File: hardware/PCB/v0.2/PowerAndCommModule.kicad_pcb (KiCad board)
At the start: 2 copper layers, 39.7 x 52.1 mm, 18 parts, among them J1 Screw_Terminal_01x02, J2 Conn_01x06_Pin, J3 Screw_Terminal_01x02, J4 Conn_01x04_Socket, J5 Screw_Terminal_01x02, K1 HF49FD_005-1H22G, Q1 S8050, SW1 SW_DIP_x01, U1 AMS1117-3.3, U2 ESP-32s

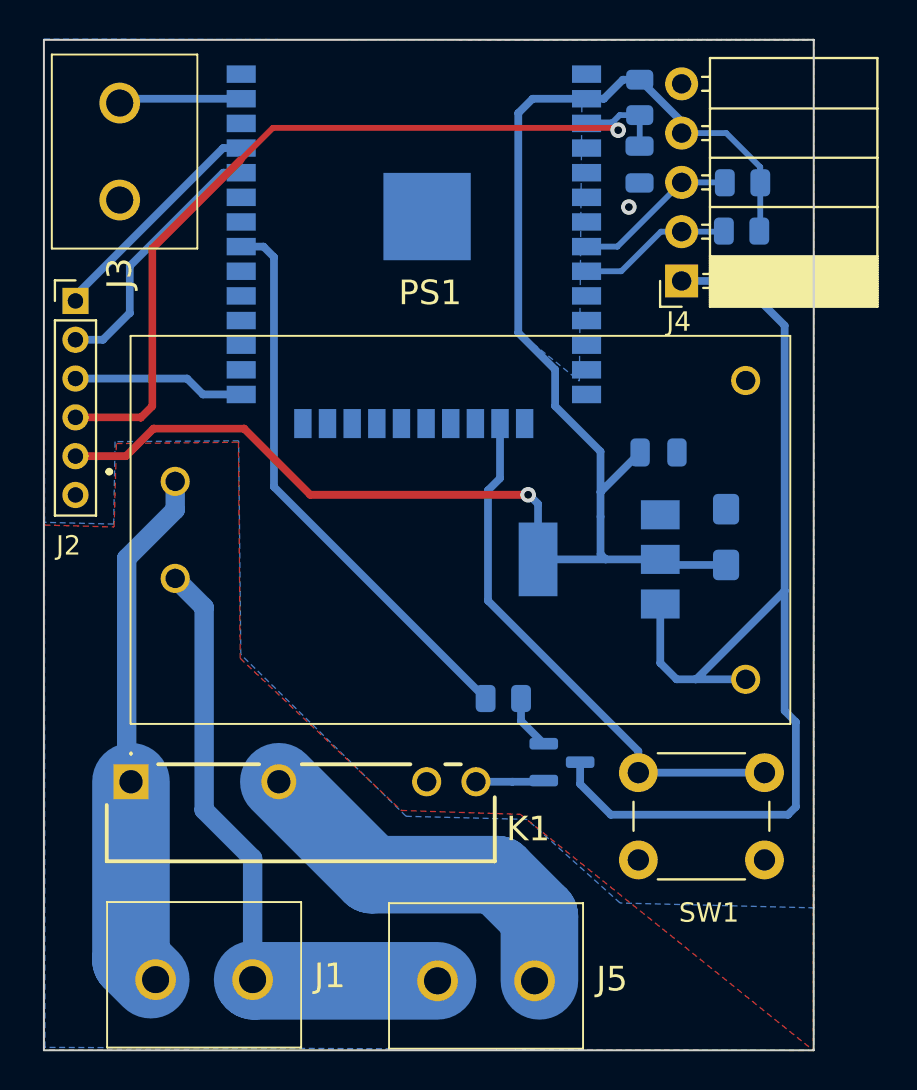
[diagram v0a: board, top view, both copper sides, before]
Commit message: commit before system update
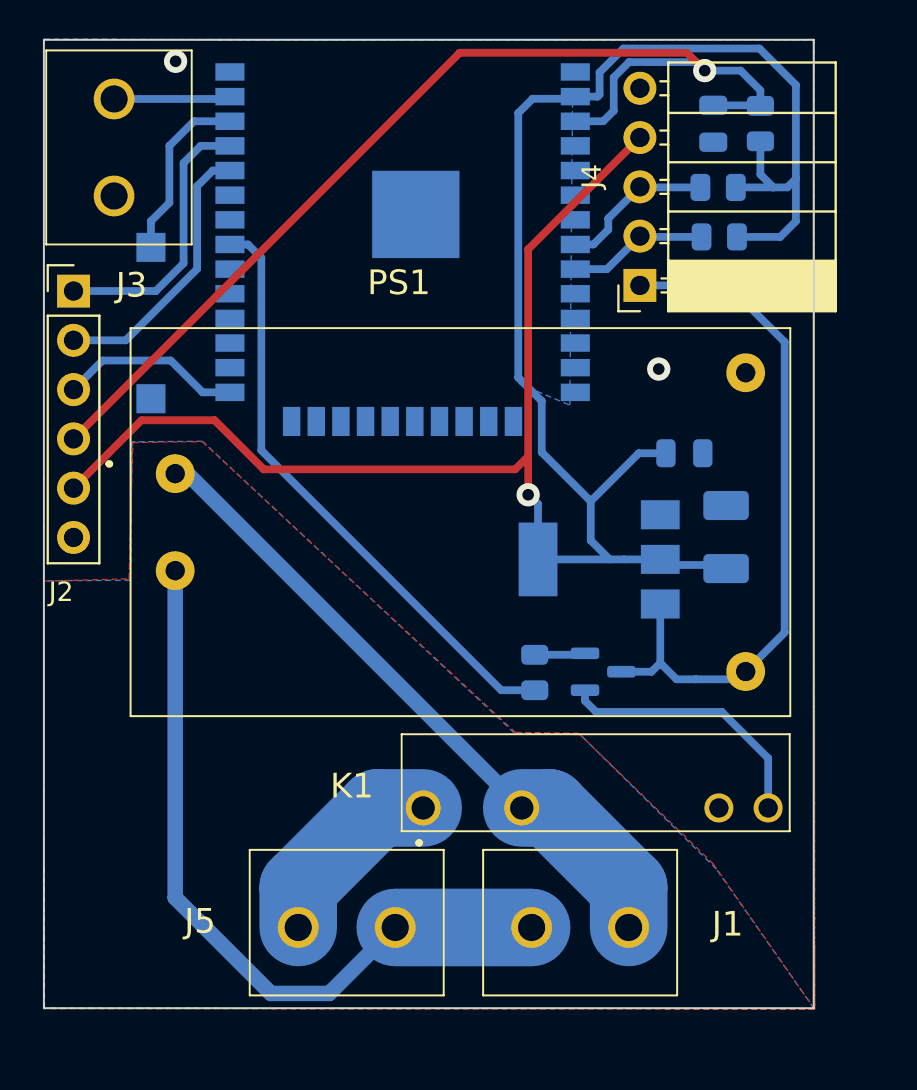
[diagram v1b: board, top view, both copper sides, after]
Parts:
- C1: footprint Capacitor_Tantalum_SMD:CP_EIA-3216-18_Kemet-A_Pad1.58x1.35mm_HandSolder -> Capacitor_Tantalum_SMD:CP_EIA-3528-21_Kemet-B_Pad1.50x2.35mm_HandSolder
- J2: footprint Connector_PinHeader_2.00mm:PinHeader_1x06_P2.00mm_Vertical -> Connector_PinHeader_2.54mm:PinHeader_1x06_P2.54mm_Vertical
- K1: value HF49FD_005-1H22G -> HF49FD_005-1H11G; footprint HF49FD_005:HF49FD0051H22G -> HF49FD_005-1H11:HF49FD0051H11F
- SW1: footprint Button_Switch_THT:SW_PUSH_6mm_H4.3mm -> Button_Switch_SMD:SW_SPST_CK_RS282G05A3; moved to B.Cu
- moved SW1 34.2 mm to (31.8, 42.6), turned to -90 degrees
- moved K1 24.0 mm to (54.7, 66.7)
- moved J1 19.6 mm to (51.4, 73.8)
- moved J5 7.69 mm to (39.4, 73.8)
- moved R1 6.36 mm to (63.2, 32.3), turned to 90 degrees
- moved Q1 5.12 mm to (55.1, 60.6)
- moved C3 4.34 mm to (60.8, 32.4)
- moved J4 2.16 mm to (57.0, 40.7)
- moved R2 2.10 mm to (51.5, 60.6), turned to 90 degrees
- moved C2 1.33 mm to (59.3, 49.3)
- moved R4 1.28 mm to (61.0, 35.6)
- moved R3 1.19 mm to (61.1, 38.2)
- moved U2 0.59 mm to (44.7, 34.9)
- moved J2 0.52 mm to (27.8, 41.0)
- moved PS1 0.40 mm to (33.0, 50.4)
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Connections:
- J1 pad 1: LINE -> NEUT
- J1 pad 2: NEUT -> LINE
- J5 pad 1: NEUT -> /LINE_NO
- J5 pad 2: /LINE_NO -> NEUT
- K1 pad 1: LINE -> /LINE_NO
- K1 pad 2: /LINE_NO -> LINE
- SW1 pad 1: Net-(U2-IO13) -> Net-(U2-IO22)
- U2 pad 16: Net-(U2-IO13) -> unconnected-(U2-IO13-Pad16)
- U2 pad 36: unconnected-(U2-IO22-Pad36) -> Net-(U2-IO22)
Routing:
- net +3V3: track 85.2 -> 124.4 mm
- net Net-(U2-IO13): track 28.0 -> 0.00 mm
- net +5V: track 58.7 -> 36.7 mm
- net /EN: track 44.0 -> 56.8 mm
- net Net-(K1-COIL_2): track 3.52 -> 13.8 mm
- net /LINE_NO: track 19.6 -> 10.2 mm
- net Net-(U2-IO22): track 0.00 -> 9.27 mm
- net LINE: track 28.6 -> 35.5 mm
- net NEUT: track 31.9 -> 38.7 mm
- net /RXD: track 12.0 -> 14.5 mm
- net Net-(U2-IO19): track 29.2 -> 31.0 mm
- net /SCL: track 7.93 -> 7.23 mm
- net /TXD: track 13.5 -> 14.2 mm
- net GND: track 0.43 -> 0.41 mm, vias 1 -> 2
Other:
- board size 39.7 x 52.1 mm -> 39.7 x 49.9 mm
